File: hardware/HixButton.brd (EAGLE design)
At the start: 54.6 x 20.1 mm, 29 parts, among them J1 FTDI, U1 ESP8266(ESP12E)V2, U2 TPS3839L30, U3 CN3058E, U4 WS2812

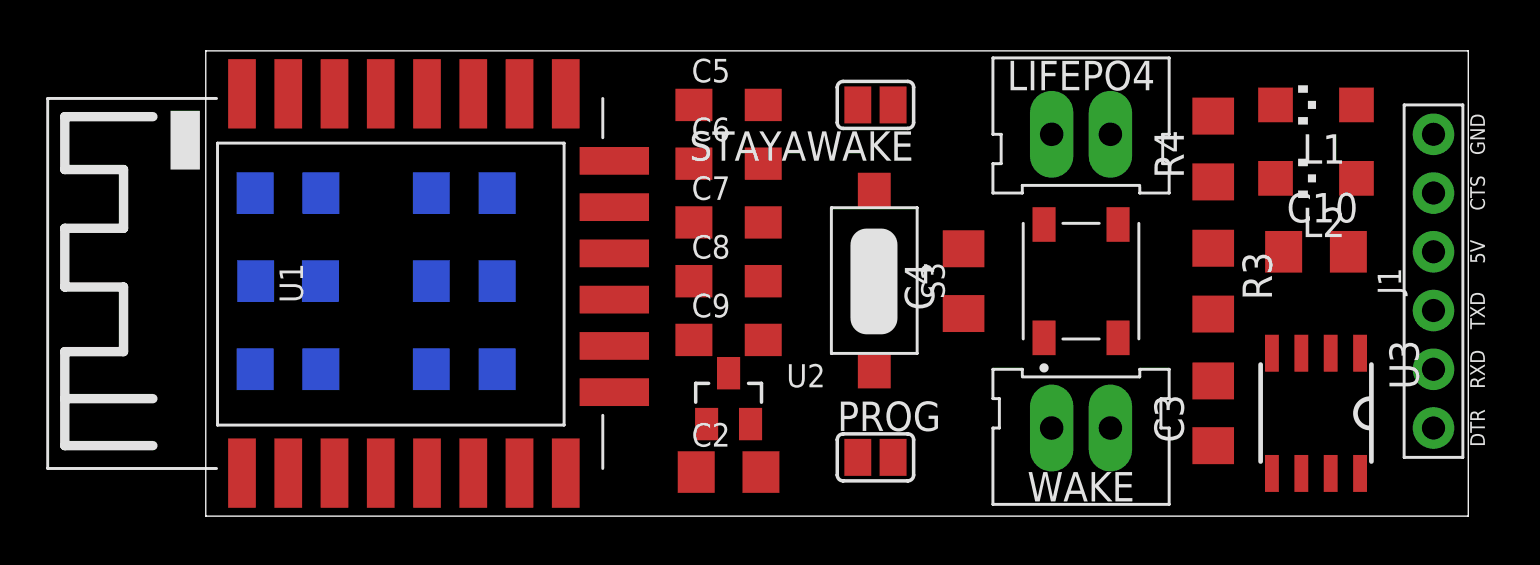
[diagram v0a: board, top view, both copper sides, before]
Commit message: update board
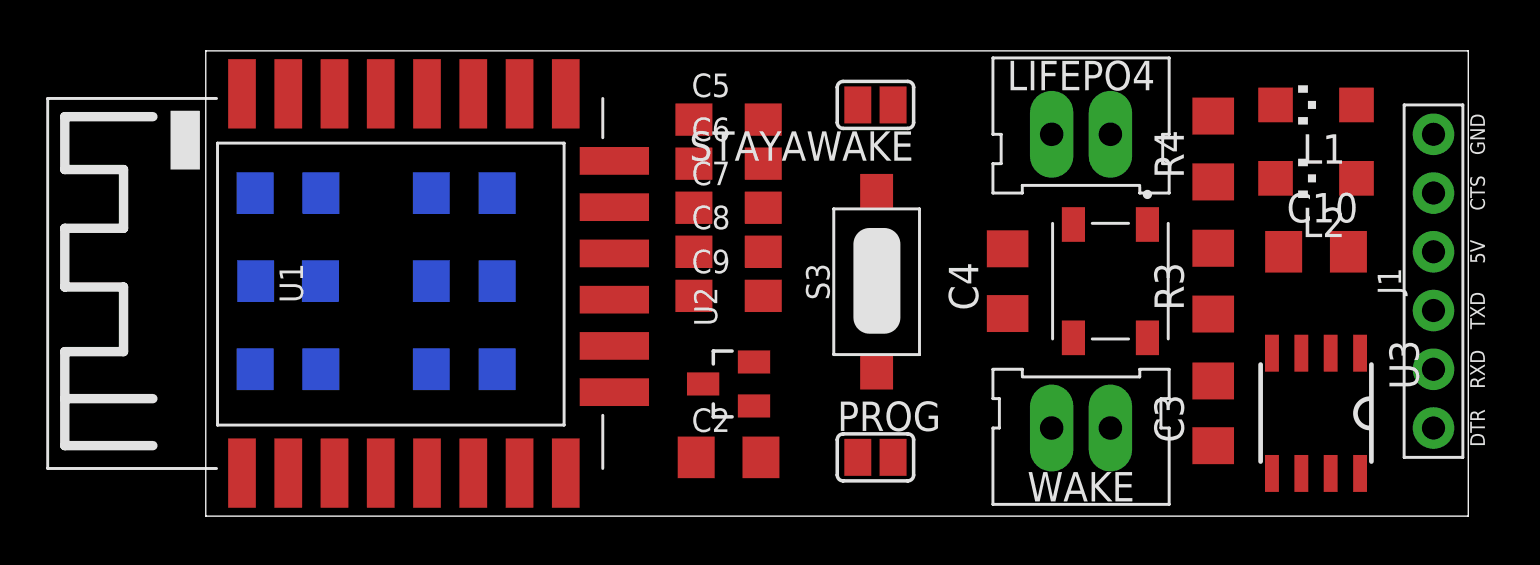
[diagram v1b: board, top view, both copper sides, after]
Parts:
- moved C4 1.91 mm to (62.9, 67.3)
- moved C9 1.91 mm to (50.8, 66.7)
- moved C8 1.27 mm to (50.8, 68.6)
- moved U4 1.27 mm to (67.3, 67.3), turned to 270 degrees
- moved C5 0.64 mm to (50.8, 74.3)
- moved C7 0.64 mm to (50.8, 70.5)
- moved U2 0.64 mm to (50.8, 62.9), turned to 90 degrees
- moved C2 0.63 mm to (50.8, 59.7)
- turned R3 to 90 degrees
- turned S3 to 90 degrees
